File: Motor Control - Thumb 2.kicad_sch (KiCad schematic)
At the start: 9 parts, among them J7 BM09B-SRSS-TB, U15 TB9051FTG,EL

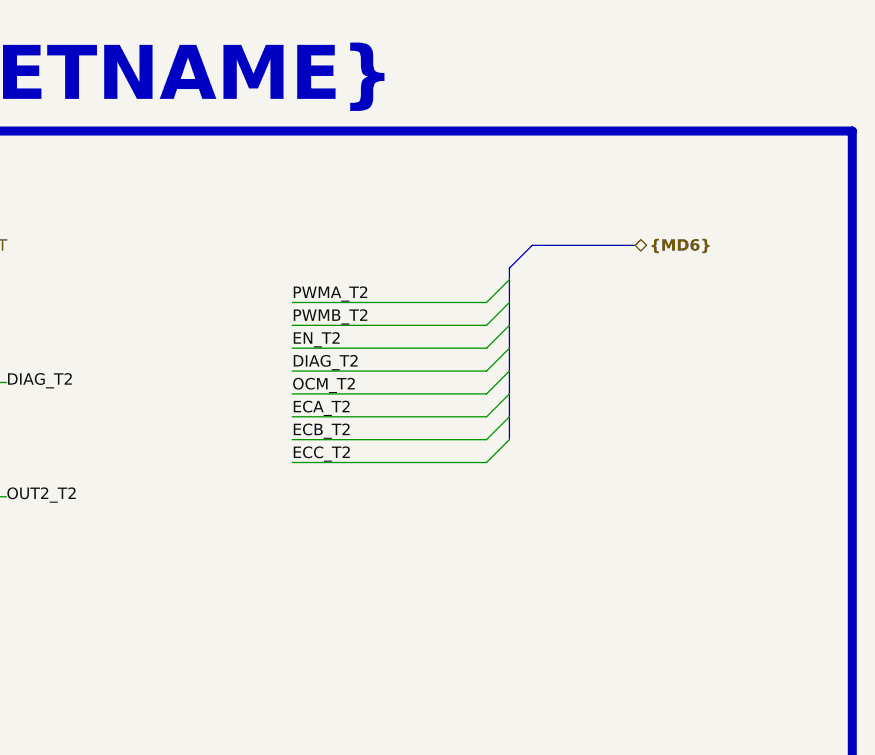
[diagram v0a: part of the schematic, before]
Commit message: Update Schematic
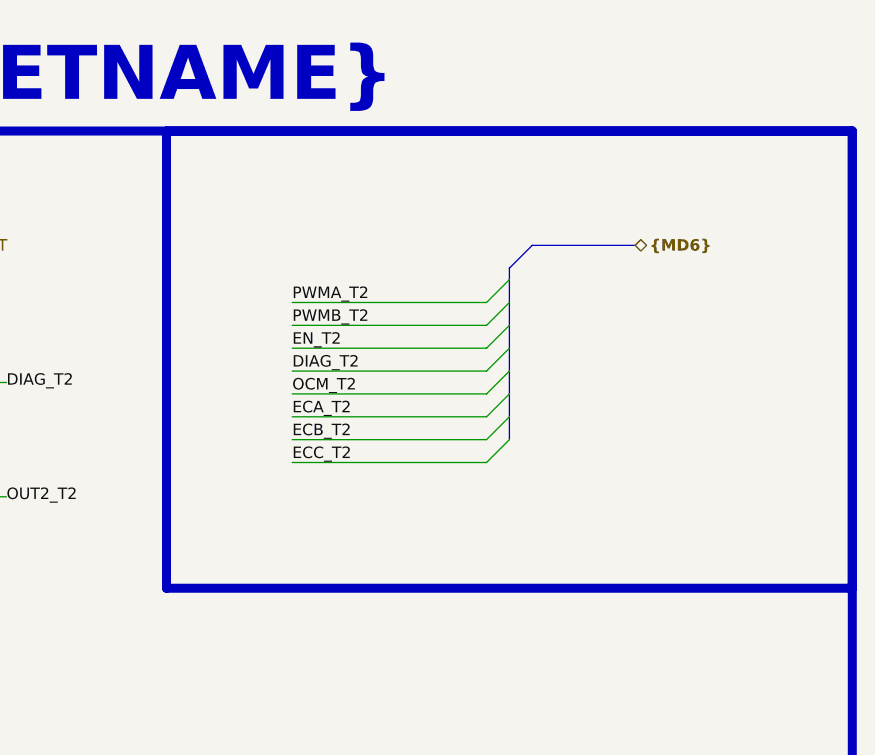
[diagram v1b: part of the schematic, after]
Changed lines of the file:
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@@
+		)
+	)
+	(rectangle
+		(start 177.8 25.4)
+		(end 254 76.2)
+		(stroke
+			(width 1)
+			(type default)
+			(color 200 0 0 1)
+		)
+		(fill
+			(type none)
 		)
 	)

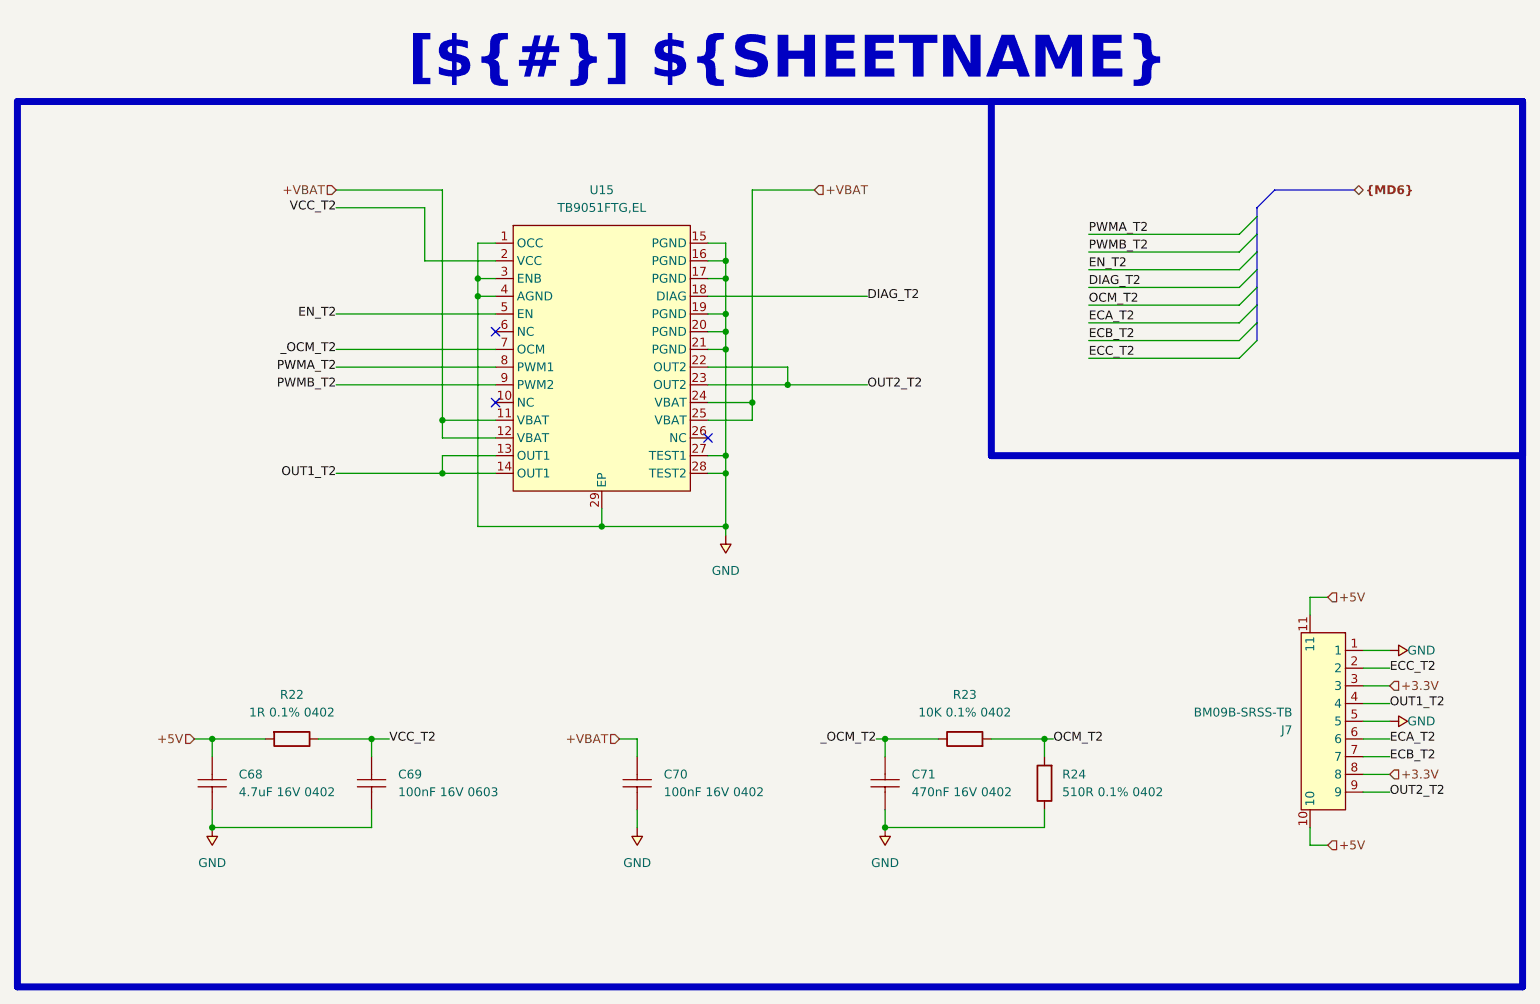
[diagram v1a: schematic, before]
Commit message: Update Schematic
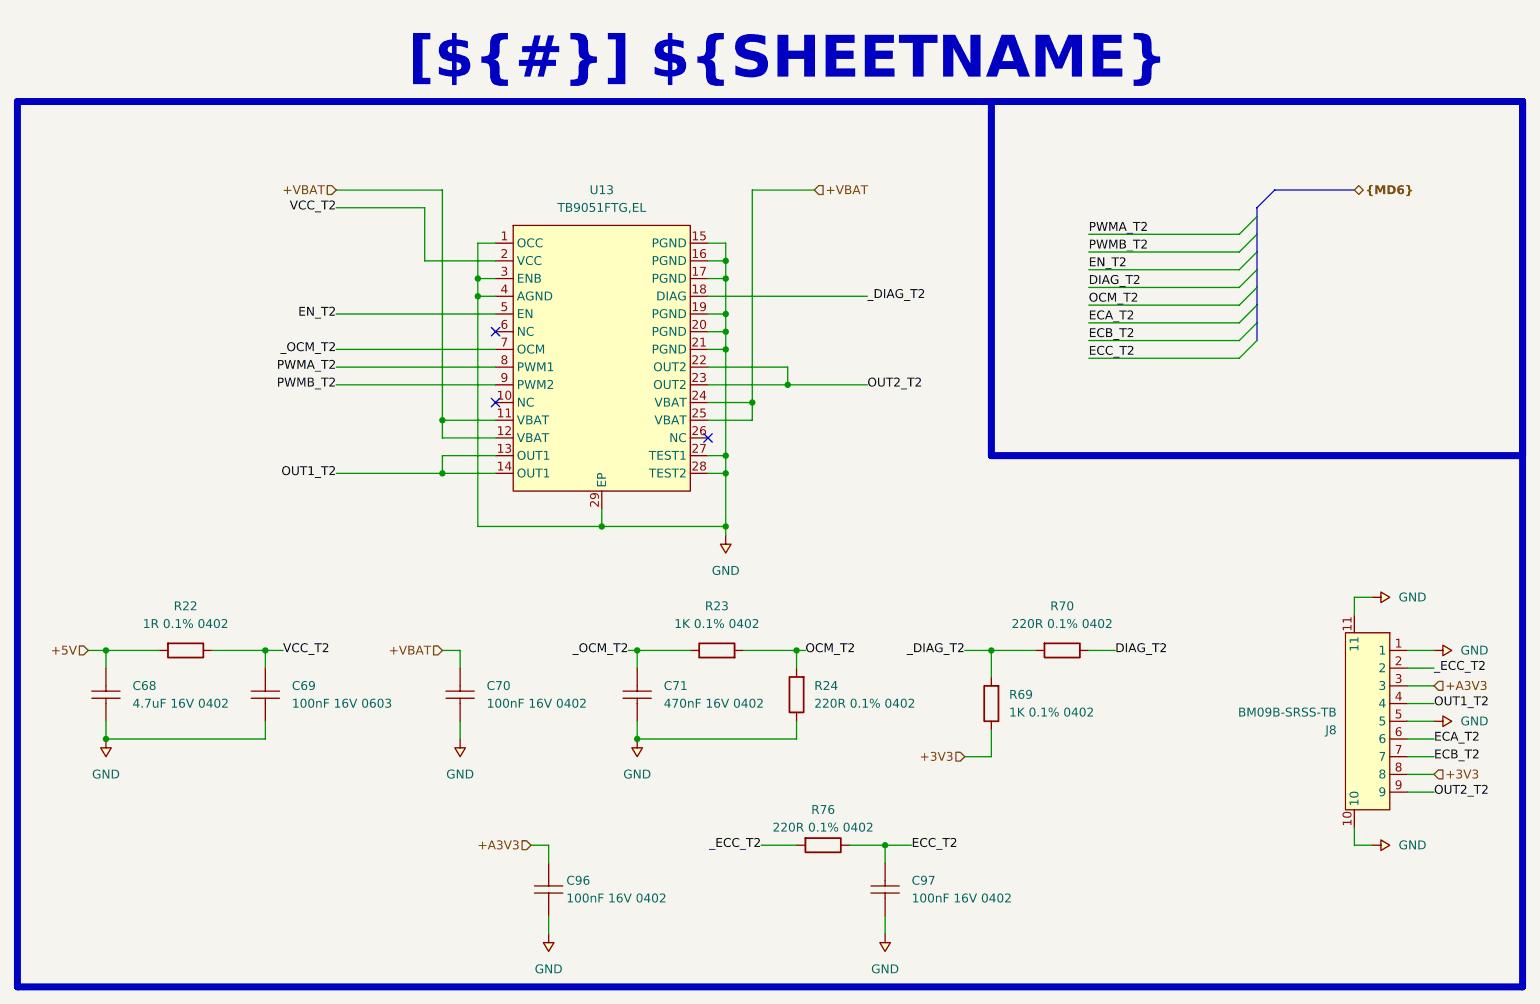
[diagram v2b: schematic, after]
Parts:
- removed J7: BM09B-SRSS-TB, Duc:CONN-SMD_9P-P1.00_BM09B-SRSS-TB, symbol Duc-Connectors:BM09B-SRSS-TB
- added C96, C97: 100nF 16V 0402, Duc_Library:C0402, symbol Duc-Capacitors:CAP CER 0402
- added J8: BM09B-SRSS-TB, Duc:CONN-SMD_9P-P1.00_BM09B-SRSS-TB, symbol Duc-Connectors:BM09B-SRSS-TB
- added R69: 1K 0.1% 0402, Duc_Library:R0402, symbol Duc-Resistors:RES SMD 0402
- added R70, R76: 220R 0.1% 0402, Duc_Library:R0402, symbol Duc-Resistors:RES SMD 0402
- R23: value 10K 0.1% 0402 -> 1K 0.1% 0402
- R24: value 510R 0.1% 0402 -> 220R 0.1% 0402
- renumbered U15 to U13
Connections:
- net DIAG_T2: now also R70.2; no longer U13.18 (DIAG)
- net ECA_T2: now also J8.6
- net ECB_T2: now also J8.7
- net ECC_T2: now also C97.2, R76.2
- net GND: now also C96.1, C97.1, J8.1, J8.10, J8.11, J8.5
- net OUT1_T2: now also J8.4
- net OUT2_T2: now also J8.9
- new net +3V3: J8.8, R69.2
- new net +A3V3: C96.2, J8.3
- new net _DIAG_T2: R69.1, R70.1, U13.18 (DIAG)
- new net _ECC_T2: J8.2, R76.1
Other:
- moved on the sheet: C68, C69, C70, C71, R22, R23, R24
